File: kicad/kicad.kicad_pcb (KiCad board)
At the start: 4 copper layers, 35 x 50 mm, 83 parts, among them J1 USB_B_Micro, J2 Conn_01x03_Pin, J3 Conn_02x10_Counter_Clockwise, J4 Conn_Coaxial_Small, SW1 RESET, SW2 BOOTSEL, U1 NCP1117-3.3_SOT223, U2 W25Q128JVS, U3 RP2040, U4 Si5351A-B-GT, U5 TRF37D73IDSGR, U6 BQ21040DBVR, Y1 ABM8-272-T3, Y2 TG2016SMN_25.0000M-MCGNNM0

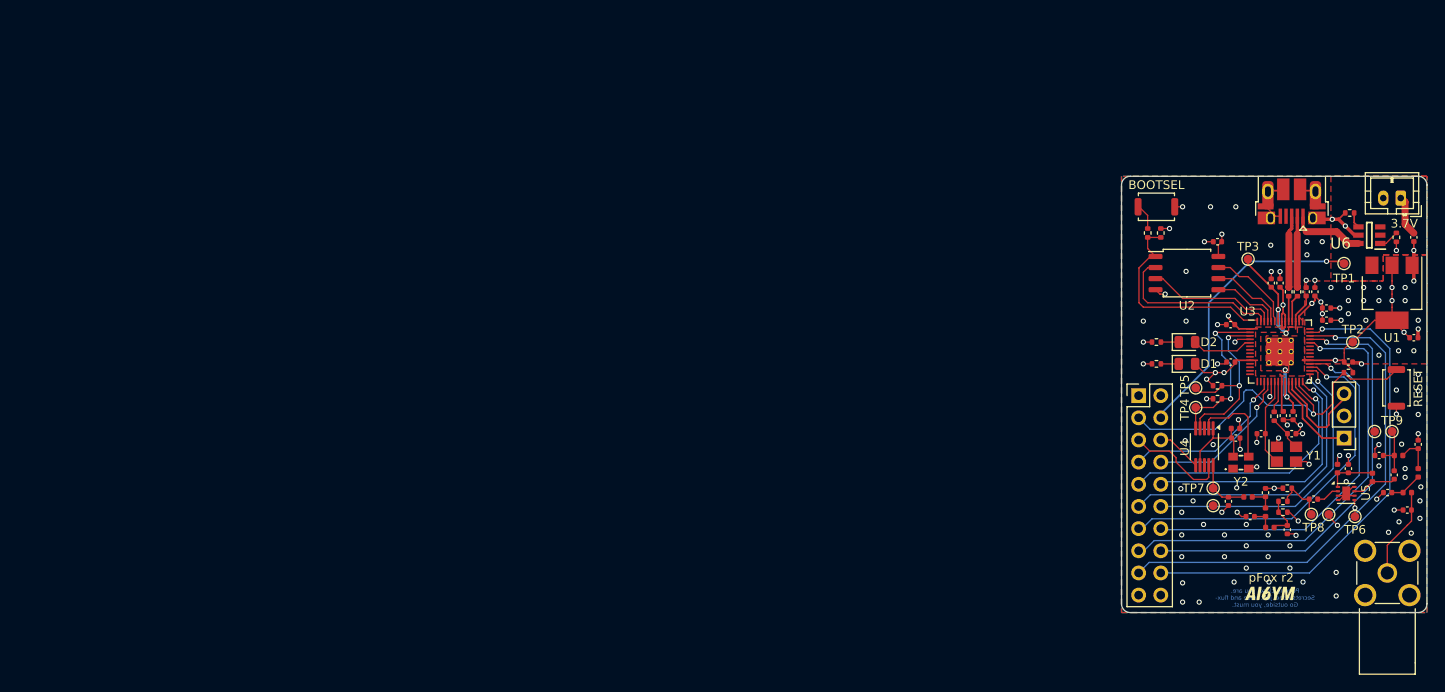
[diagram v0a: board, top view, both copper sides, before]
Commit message: PicoFox r3
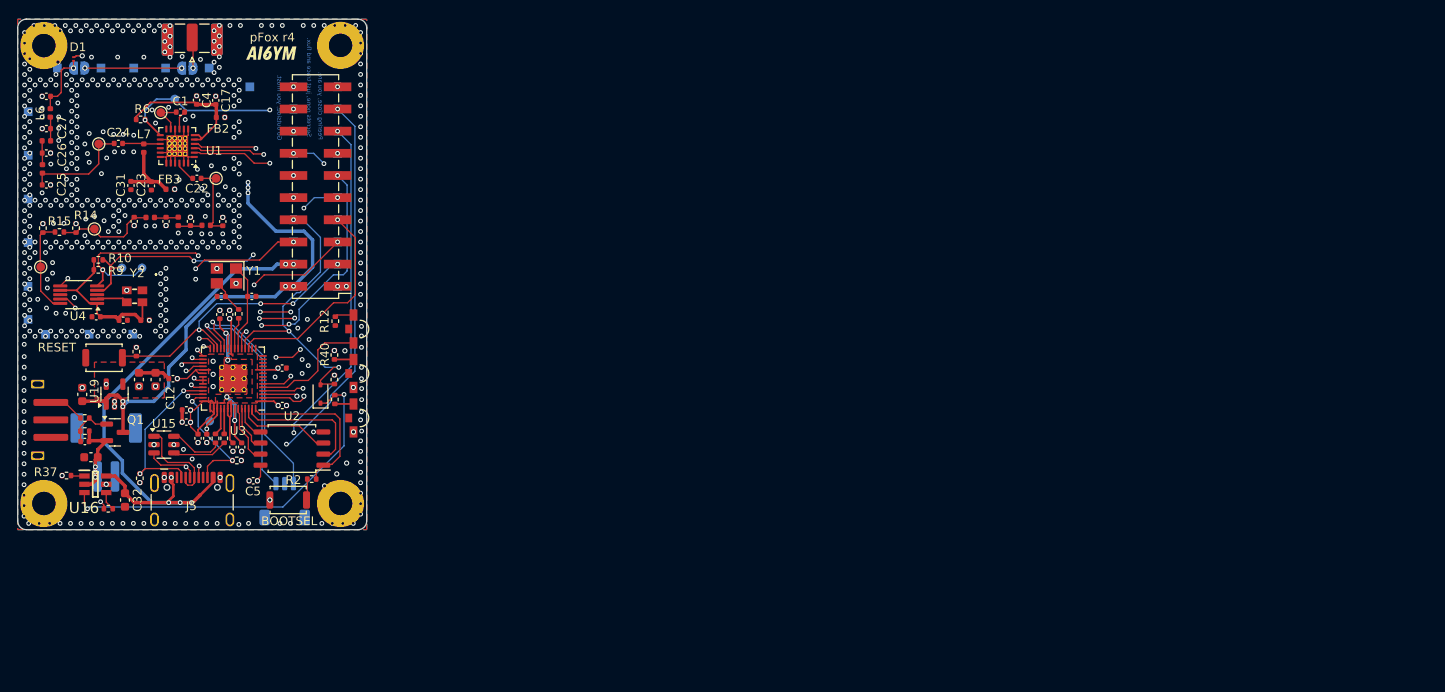
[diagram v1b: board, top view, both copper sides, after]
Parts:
- removed BT1: 3.7V, Connector_JST:JST_PH_B2B-PH-K_1x02_P2.00mm_Vertical
- removed J1: USB_B_Micro, RP2040_minimal:USB_Micro-B_Amphenol_10103594-0001LF_Horizontal_modified
- removed R11: 300, Resistor_SMD:R_0402_1005Metric
- removed TP12, TP13: TestPoint, TestPoint:TestPoint_Pad_D1.0mm
- removed U5: TRF37D73IDSGR, Package_SON:WSON-8-1EP_2x2mm_P0.5mm_EP0.9x1.6mm
- removed U6: BQ21040DBVR, AI6YM:SOT95P280X145-6N
- added BT2: 3.7V, PicofoxLib:JST PH 2 Horizontal, B.Cu at (60.1, 105.9)
- added C29: 10uF, Capacitor_SMD:C_0603_1608Metric, F.Cu at (58.4, 103.7)
- added C30: 10uF, Capacitor_SMD:C_0603_1608Metric, F.Cu at (63.9, 94.8)
- added C31: 100nF, Capacitor_SMD:C_0402_1005Metric, F.Cu at (63.0, 72.6)
- added C32: 10uF, Capacitor_SMD:C_0603_1608Metric, F.Cu at (62.3, 108.6)
- added C33: 100nF, Capacitor_SMD:C_0402_1005Metric, F.Cu at (57.7, 101.9)
- added C40: 10uF, Capacitor_SMD:C_0603_1608Metric, F.Cu at (65.8, 94.8)
- added C58: 10uF, Capacitor_SMD:C_0603_1608Metric, F.Cu at (57.4, 96.5)
- added C67: 100nF, Capacitor_SMD:C_0402_1005Metric, F.Cu at (59.0, 87.6)
- added C68: 100pF, Capacitor_SMD:C_0402_1005Metric, F.Cu at (62.1, 88.0)
- added D3: 1N4148WS, Diode_SMD:D_SOD-323, F.Cu at (84.7, 96.5)
- added D4: LED, PicofoxLib:LED 1206 Side View, F.Cu at (88.5, 99.2)
- added D5: LED, PicofoxLib:LED 1206 Side View, F.Cu at (88.5, 94.1)
- added FB3: 600, Inductor_SMD:L_0402_1005Metric, F.Cu at (67.5, 73.0)
- added H1: MountingHole, MountingHole:MountingHole_2.7mm_M2.5_Pad, F.Cu at (53.0, 56.5)
- added H2: MountingHole, MountingHole:MountingHole_2.7mm_M2.5_Pad, F.Cu at (87.0, 56.5)
- added H3: MountingHole, MountingHole:MountingHole_2.7mm_M2.5_Pad, F.Cu at (53.0, 109.0)
- added H4: MountingHole, MountingHole:MountingHole_2.7mm_M2.5_Pad, F.Cu at (87.0, 109.0)
- added J5: USB-TYPE-C-018 (DEALON), PicofoxLib:USB_C_Receptacle_HCTL_HC-TYPE-C-16P-01A, F.Cu at (70.0, 109.4)
- added JP1: SolderJumper_2_Open, Jumper:SolderJumper-2_P1.3mm_Open_RoundedPad1.0x1.5mm, B.Cu at (57.0, 59.1)
- added JP2: SolderJumper_2_Open, Jumper:SolderJumper-2_P1.3mm_Open_RoundedPad1.0x1.5mm, B.Cu at (69.5, 59.1)
- added Q1: AO3407A, Package_TO_SOT_SMD:SOT-23, F.Cu at (61.1, 100.8)
- added R27: 5.11KR, Resistor_SMD:R_0402_1005Metric, F.Cu at (75.1, 104.1)
- added R28: 5.11KR, Resistor_SMD:R_0402_1005Metric, F.Cu at (64.0, 106.1)
- added R36: 1KR, Resistor_SMD:R_0402_1005Metric, F.Cu at (60.4, 109.6)
- added R37: 10KR, Resistor_SMD:R_0402_1005Metric, F.Cu at (55.6, 105.8)
- added R38: 10KR, Resistor_SMD:R_0402_1005Metric, F.Cu at (86.3, 94.8)
- added R39: 294R, Resistor_SMD:R_0402_1005Metric, F.Cu at (86.3, 97.1)
- added R40: 120R, Resistor_SMD:R_0402_1005Metric, F.Cu at (86.3, 92.0)
- added SW3: SK-12D15-G030, PicofoxLib:SW_Slide_SPDT_Angled_CK_OS102011MA1Q, F.Cu at (52.3, 99.4)
- added TP17: TestPoint, PicofoxLib:Castellation Pad, B.Cu at (86.7, 81.6)
- added TP19: TestPoint, PicofoxLib:Castellation Pad, B.Cu at (86.7, 79.0)
- added TP20: TestPoint, PicofoxLib:Castellation Pad, B.Cu at (86.7, 76.5)
- added TP21: TestPoint, PicofoxLib:Castellation Pad, B.Cu at (86.7, 74.0)
- added TP22: TestPoint, PicofoxLib:Castellation Pad, B.Cu at (86.7, 71.4)
- added TP23: TestPoint, PicofoxLib:Castellation Pad, B.Cu at (86.7, 68.9)
- added TP24: TestPoint, PicofoxLib:Castellation Pad, B.Cu at (81.6, 61.2)
- added TP25: TestPoint, PicofoxLib:Castellation Pad, B.Cu at (86.7, 63.8)
- added TP26: TestPoint, PicofoxLib:Castellation Pad, B.Cu at (86.7, 66.3)
- added TP27: TestPoint, PicofoxLib:Castellation Pad, B.Cu at (86.7, 61.2)
- added TP28: TestPoint, PicofoxLib:Castellation Pad, B.Cu at (81.6, 63.8)
- added TP29: TestPoint, PicofoxLib:Castellation Pad, B.Cu at (81.6, 66.3)
- added TP30: TestPoint, PicofoxLib:Castellation Pad, B.Cu at (81.6, 68.9)
- added TP31: TestPoint, PicofoxLib:Castellation Pad, B.Cu at (81.6, 71.4)
- added TP32: TestPoint, PicofoxLib:Castellation Pad, B.Cu at (81.6, 74.0)
- added TP33: TestPoint, PicofoxLib:Castellation Pad, B.Cu at (81.6, 76.5)
- added TP34: TestPoint, PicofoxLib:Castellation Pad, B.Cu at (81.6, 79.0)
- added TP35: TestPoint, PicofoxLib:Castellation Pad, B.Cu at (81.6, 81.6)
- added TP36: TestPoint, PicofoxLib:Castellation Pad, B.Cu at (81.6, 84.1)
- added TP37: TestPoint, PicofoxLib:Castellation Pad, B.Cu at (54.5, 59.1)
- added TP38: TestPoint, PicofoxLib:Castellation Pad, B.Cu at (59.5, 59.1)
- added TP39: TestPoint, PicofoxLib:Castellation Pad, B.Cu at (67.0, 59.1)
- added TP40: TestPoint, PicofoxLib:Castellation Pad, B.Cu at (72.0, 59.1)
- added TP41: TestPoint, PicofoxLib:Castellation Pad, B.Cu at (53.2, 89.6)
- added TP42: TestPoint, PicofoxLib:Castellation Pad, B.Cu at (51.2, 69.1)
- added TP43: TestPoint, PicofoxLib:Castellation Pad, B.Cu at (51.2, 74.1)
- added TP44: TestPoint, PicofoxLib:Castellation Pad, B.Cu at (63.3, 59.1)
- added TP45: TestPoint, PicofoxLib:Castellation Pad, B.Cu at (51.2, 84.1)
- added TP46: TestPoint, PicofoxLib:Castellation Pad, B.Cu at (76.6, 61.2)
- added TP47: TestPoint, PicofoxLib:Castellation Pad, B.Cu at (58.2, 89.6)
- added TP48: TestPoint, PicofoxLib:Castellation Pad, B.Cu at (51.2, 79.1)
- added TP49: TestPoint, PicofoxLib:Castellation Pad, B.Cu at (51.2, 64.1)
- added TP51: TestPoint, PicofoxLib:Castellation Pad, B.Cu at (63.2, 89.6)
- added TP53: TestPoint, PicofoxLib:Castellation Pad, B.Cu at (51.2, 87.9)
- added U15: USBLC6-2SC6, Package_TO_SOT_SMD:SOT-23-6, F.Cu at (66.8, 102.2)
- added U16: BQ21040DBVR, PicofoxLib:SOT95P280X145-6N, F.Cu at (58.9, 106.8)
- added U19: ME6217C33M5G, Package_TO_SOT_SMD:SOT-23-5, F.Cu at (61.1, 96.5)
- C1: value 10u -> 10nF
- C10, C8: value 1u -> 1uF
- C11, C12, C13, C14, C15, C16, C5, C6, C7, C9: value 100n -> 100nF
- C17: value 10u -> 100nF
- C18, C21, C25, C28: value 24p -> 24pF
- C19, C20, C26, C27: value 43p -> 43pF
- C2, C3: value 15p -> 15pF
- C22, C24: value 1n -> 10nF
- C23, C4: value 10u -> 100pF
- D1: value LED -> H5VU06B; footprint LED_SMD:LED_0805_2012Metric -> PicofoxLib:DFN0603-2L
- D2: footprint LED_SMD:LED_0805_2012Metric -> PicofoxLib:LED 1206 Side View
- G***, TP3, TP4, TP5, TP6: moved to B.Cu
- J2: footprint Connector_PinHeader_2.54mm:PinHeader_1x03_P2.54mm_Vertical -> Connector_JST:JST_SH_SM03B-SRSS-TB_1x03-1MP_P1.00mm_Horizontal; moved to B.Cu
- J3: footprint Connector_PinHeader_2.54mm:PinHeader_2x10_P2.54mm_Vertical -> Connector_PinHeader_2.54mm:PinHeader_2x10_P2.54mm_Vertical_SMD
- J4: footprint AI6YM:SMA_HORIZONTAL -> Connector_Coaxial:SMA_Samtec_SMA-J-P-H-ST-EM1_EdgeMount
- L1, L3, L4, L6: value 68n -> 68nH
- L2, L5: value 75n -> 75nH
- L7: renamed from FB3; value 600 -> 270nH
- R1: value 1k -> 100KR
- R10, R9: value 2.2k -> 2.2KR
- R12: value 300 -> 120R
- R13, R14: value 36 -> 294R
- R15: value 150 -> 17.4R
- R2: value DNF -> 10KR
- R3, R4: value 27 -> 33R
- R5, R7: value 1k -> 1KR
- R6: value 10k -> 1KR
- R8: value 10k -> 10KR
- SW1: value RESET -> ~
- SW2: value BOOTSEL -> ~
- TP14: footprint TestPoint:TestPoint_Pad_D1.0mm -> PicofoxLib:Castellation Pad; moved to B.Cu
- U1: value NCP1117-3.3_SOT223 -> BVA1761; footprint Package_TO_SOT_SMD:SOT-223-3_TabPin2 -> Package_DFN_QFN:QFN-24-1EP_4x4mm_P0.5mm_EP2.5x2.5mm
- moved C28 163.0 mm to (53.3, 62.3)
- moved L5 161.7 mm to (53.3, 67.4), turned to 0 degrees
- moved L6 161.5 mm to (53.7, 64.2), turned to 90 degrees
- moved C26 160.7 mm to (53.3, 68.8), turned to 0 degrees
- moved C27 159.3 mm to (53.3, 66.0)
- moved L4 158.8 mm to (52.8, 70.7), turned to 90 degrees
- moved C25 155.8 mm to (53.3, 72.5), turned to 0 degrees
- moved TP9 151.8 mm to (59.3, 67.8), turned to 180 degrees
- moved C24 151.1 mm to (61.5, 67.7), turned to 180 degrees
- moved J4 150.1 mm to (70.0, 55.6), turned to 90 degrees
- moved SW1 148.1 mm to (59.9, 92.3), turned to 0 degrees
- moved R7 146.8 mm to (57.7, 99.2)
- moved R13 145.8 mm to (52.9, 77.4), turned to 90 degrees
- moved L7 145.8 mm to (64.5, 68.3), turned to -90 degrees
- moved TP2 144.8 mm to (58.8, 77.5), turned to 180 degrees
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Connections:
- net /GPIO15 renamed /ChgSense
- net /GPIO27_ADC1 renamed /CC1Sense
- net /GPIO29_ADC3 renamed /CC2Sense
- net /PostS1-TLINE renamed Net-(C26-Pad1)
- net /PostS2-TLINE renamed Net-(C27-Pad1)
- net /PreS1-TLINE renamed Net-(C19-Pad1)
- net /PreS2-TLINE renamed Net-(C20-Pad1)
- net /ToPost-TLINE renamed Net-(C24-Pad2)
- C1 pad 1: +BATT -> Net-(U1-RF2)
- C1 pad 2: GND -> Net-(U1-RF3)
- C17 pad 2: Net-(U4-VDD) -> Net-(U1-DSAVDD)
- C18 pad 1: /SIGGEN-TLINE -> Net-(C18-Pad1)
- C21 pad 1: /ToAmp-TLINE -> Net-(C21-Pad1)
- C22 pad 1: Net-(C22-Pad1) -> Net-(C21-Pad1)
- C22 pad 2: /AMPIN-TLINE -> Net-(U1-RF1)
- C23 pad 2: Net-(U5-VCC) -> Net-(C23-Pad2)
- C24 pad 1: /AMP-TLINE -> Net-(U1-RF4)
- C28 pad 1: /ToAnt-TLINE -> Net-(D1-A2)
- C4 pad 1: +3V3 -> GND
- C4 pad 2: GND -> Net-(U1-DSAVDD)
- D1 pad 1: Net-(D1-K) -> GND
- D1 pad 2: +3V3 -> Net-(D1-A2)
- D2 pad 1: Net-(D2-K) -> Net-(D2-A)
- D2 pad 2: Net-(D2-A) -> Net-(D2-K)
- FB2 pad 2: Net-(U5-VCC) -> Net-(U1-DSAVDD)
- J3 pad 2: +3V3 -> /SWITCHED_VBATT
- J3 pad 4: +BATT -> VBUS
- J4 pad 1: /ToAnt-TLINE -> Net-(J4-In)
- L1 pad 1: /SIGGEN-TLINE -> Net-(C18-Pad1)
- L3 pad 2: /ToAmp-TLINE -> Net-(C21-Pad1)
- L6 pad 2: /ToAnt-TLINE -> Net-(D1-A2)
- L7 pad 1: /AMP-TLINE -> Net-(U1-RF4)
- L7 pad 2: Net-(U5-VCC) -> Net-(C23-Pad2)
- R1 pad 1: /QSPI_SS -> +BATT
- R1 pad 2: /~{USB_BOOT} -> Net-(Q1-G)
- R10 pad 2: +3V3 -> Net-(U4-VDD)
- R13 pad 1: /ToAmp-TLINE -> Net-(U4-CLK0)
- R14 pad 1: Net-(C22-Pad1) -> Net-(C18-Pad1)
- R15 pad 1: /ToAmp-TLINE -> Net-(U4-CLK0)
- R15 pad 2: Net-(C22-Pad1) -> Net-(C18-Pad1)
- R2 pad 1: +3V3 -> /~{USB_BOOT}
- R6 pad 1: Net-(U6-TS) -> /AMP_EN
- R6 pad 2: GND -> Net-(U1-DSAVDD)
- R7 pad 1: Net-(U6-ISET) -> Net-(Q1-G)
- R7 pad 2: GND -> Net-(SW3-A)
- R9 pad 2: +3V3 -> Net-(U4-VDD)
- TP1 pad 1: +BATT -> Net-(U1-RF3)
- TP14 pad 1: GND -> +3V3
- TP2 pad 1: +3V3 -> Net-(C18-Pad1)
- TP7 pad 1: /SIGGEN-TLINE -> Net-(U4-CLK0)
- TP8 pad 1: Net-(C22-Pad1) -> Net-(C21-Pad1)
- U1 pad 2: +3V3 -> /ATTN_LE
- U1 pad 3: +BATT -> /I2C0 SCL
- U3 pad 34: unconnected-(U3-GPIO22-Pad34) -> +3V3
- U3 pad 35: unconnected-(U3-GPIO23-Pad35) -> GND
- U3 pad 36: unconnected-(U3-GPIO24-Pad36) -> GND
- U3 pad 37: unconnected-(U3-GPIO25-Pad37) -> GND
- U3 pad 6: unconnected-(U3-GPIO4-Pad6) -> /ATTN_LE
- U4 pad 10: /SIGGEN-TLINE -> Net-(U4-CLK0)
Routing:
- net VBUS: track 0.00 -> 92.7 mm, vias 0 -> 8
- net /SWITCHED_VBATT: track 0.00 -> 66.2 mm, vias 0 -> 8
- net /I2C0 SDA: track 19.0 -> 70.7 mm, vias 2 -> 5
- net /I2C0 SCL: track 22.2 -> 71.8 mm, vias 2 -> 5
- net Net-(D3-K): track 0.00 -> 43.4 mm, vias 0 -> 2
- net /ATTN_LE: track 0.00 -> 38.2 mm, vias 0 -> 2
- net +BATT: track 38.0 -> 9.87 mm, vias 1 -> 3
- net /CLK1: track 11.7 -> 39.5 mm, vias 0 -> 3
- net GND: track 64.7 -> 36.9 mm, vias 91 -> 522
- net /AMP_EN: track 29.9 -> 57.2 mm, vias 2 -> 3
- net /GPIO20: track 42.1 -> 66.7 mm, vias 1 -> 2
- net /CLK2: track 5.20 -> 29.6 mm, vias 0 -> 3
- net +3V3: track 65.7 -> 41.8 mm, vias 32 -> 20
- net /GPIO21: track 42.3 -> 64.7 mm, vias 1 -> 3
- net /CC1Sense: track 50.5 -> 71.7 mm, vias 1 -> 3
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- removed copper zone on F.Cu, net +BATT
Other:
- board size 35 x 50 mm -> 40 x 58.5 mm
- board text added: "+ -"
- board text added: "1.1V"
- board text added: "AMP_EN"
- board text added: "BOOTSEL"
- board text added: "Go outside, you must."
- board text added: "Peering close, you are."
- board text added: "RESET"
- board text added: "SDA SCL"
- board text added: "Secrets none, just trace and flux."
- board text added: "pFox r4"
- board text removed: "3.3v"
- board text removed: "3.7V"
- board text removed: "BATT/RUN"
- board text removed: "CLK2/CLK1"
- board text removed: "GND"
- board text removed: "GP15/14"
- board text removed: "GP17/16"
- board text removed: "GP19/18"
- board text removed: "GP21/20"
- board text removed: "GP27/26(A)"
- board text removed: "GP29/28(A)"
- board text removed: "Peering close, you are. Secrets none, just trace and flux- Go outside, you must."
- board text removed: "SWCLK"
- board text removed: "pFox r2"
